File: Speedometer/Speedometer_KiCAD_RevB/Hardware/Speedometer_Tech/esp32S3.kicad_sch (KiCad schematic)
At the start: 34 parts, among them J2 Conn_01x08_Pin, Q601 DTC123J, Q602 DTC123J, U601 ESP32-S3-WROOM-1(N8R2), U602 BC817, U603 CP2102N-A02-GQFN28R, U604 BC817, U605 YTC-TC16S-24

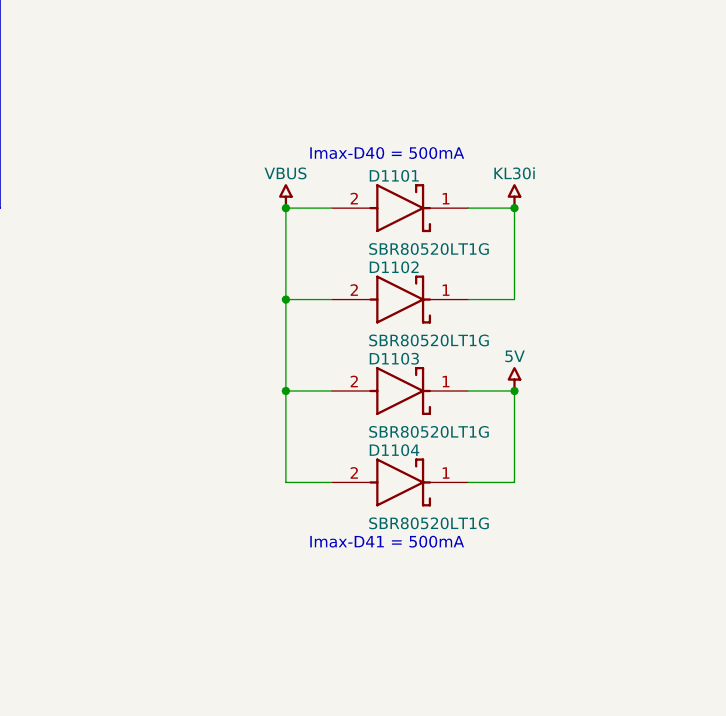
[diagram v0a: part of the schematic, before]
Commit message: pcb should be done now
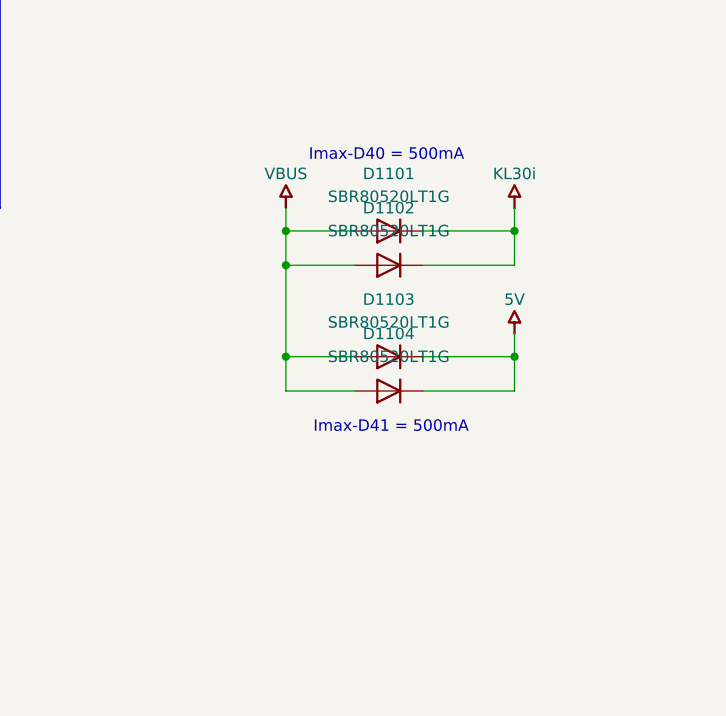
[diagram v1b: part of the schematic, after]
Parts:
- removed D1101, D1102, D1103, D1104: SBR80520LT1G, FP-425-04-MFG, symbol Speedometer_Tech-altium-import:Designator_0_1d6ec82d83fb6aee721767c19dac4b9
- added D1101, D1102, D1103, D1104: SBR80520LT1G, Diode_SMD:D_SOD-123, symbol Device:D
- C604: footprint footprint:C0603 -> Capacitor_SMD:C_0603_1608Metric
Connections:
- net 5V: now also D1103.1 (K), D1104.1 (K)
- net KL30i: now also D1101.1 (K), D1102.1 (K)
- net VBUS: now also D1101.2 (A), D1102.2 (A), D1103.2 (A), D1104.2 (A)
